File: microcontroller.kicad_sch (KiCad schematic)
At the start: 65 parts, among them IC1 MIMXRT1062DVJ6B, J3 503182-1852, J4 USB_C_pycubed, J5 JTAG_SWD_10, J6 Conn_01x06, Q6 DMG2305UX-7, SW1 KMR231NG LFS, U6 TPS54226PWPR, U7 MR25H40MDF, U8 MKL02Z32VFG4, Y1 24.0mHz, Y2 32.768kHz

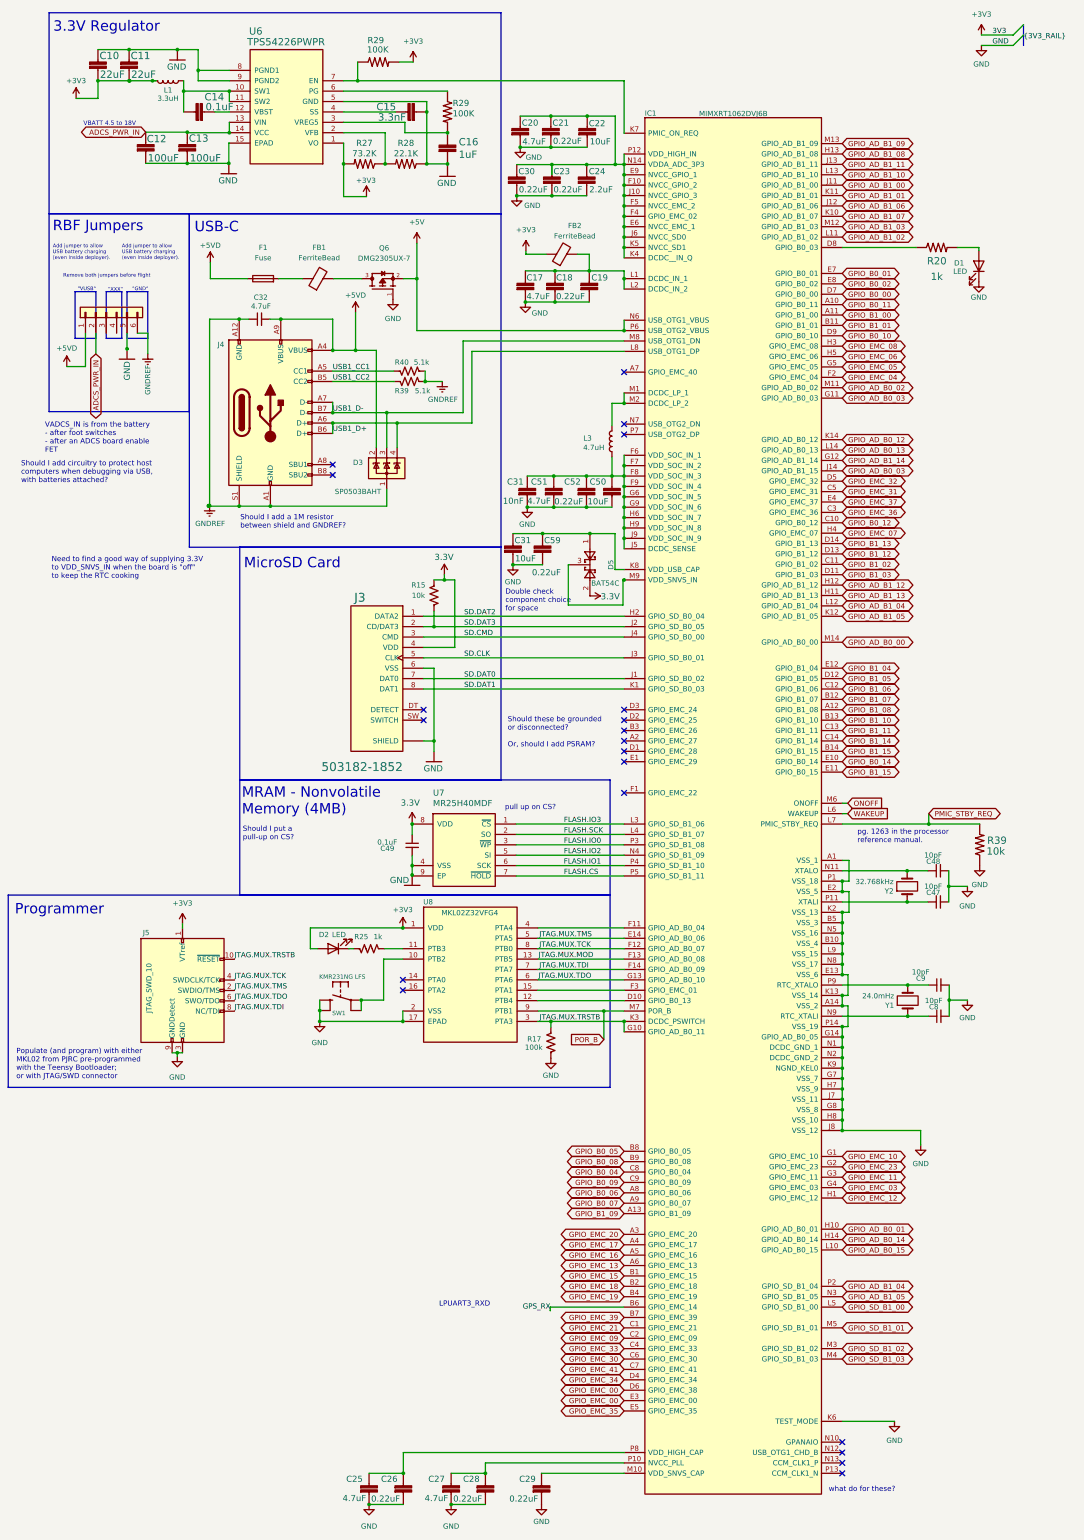
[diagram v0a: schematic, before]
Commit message: organize
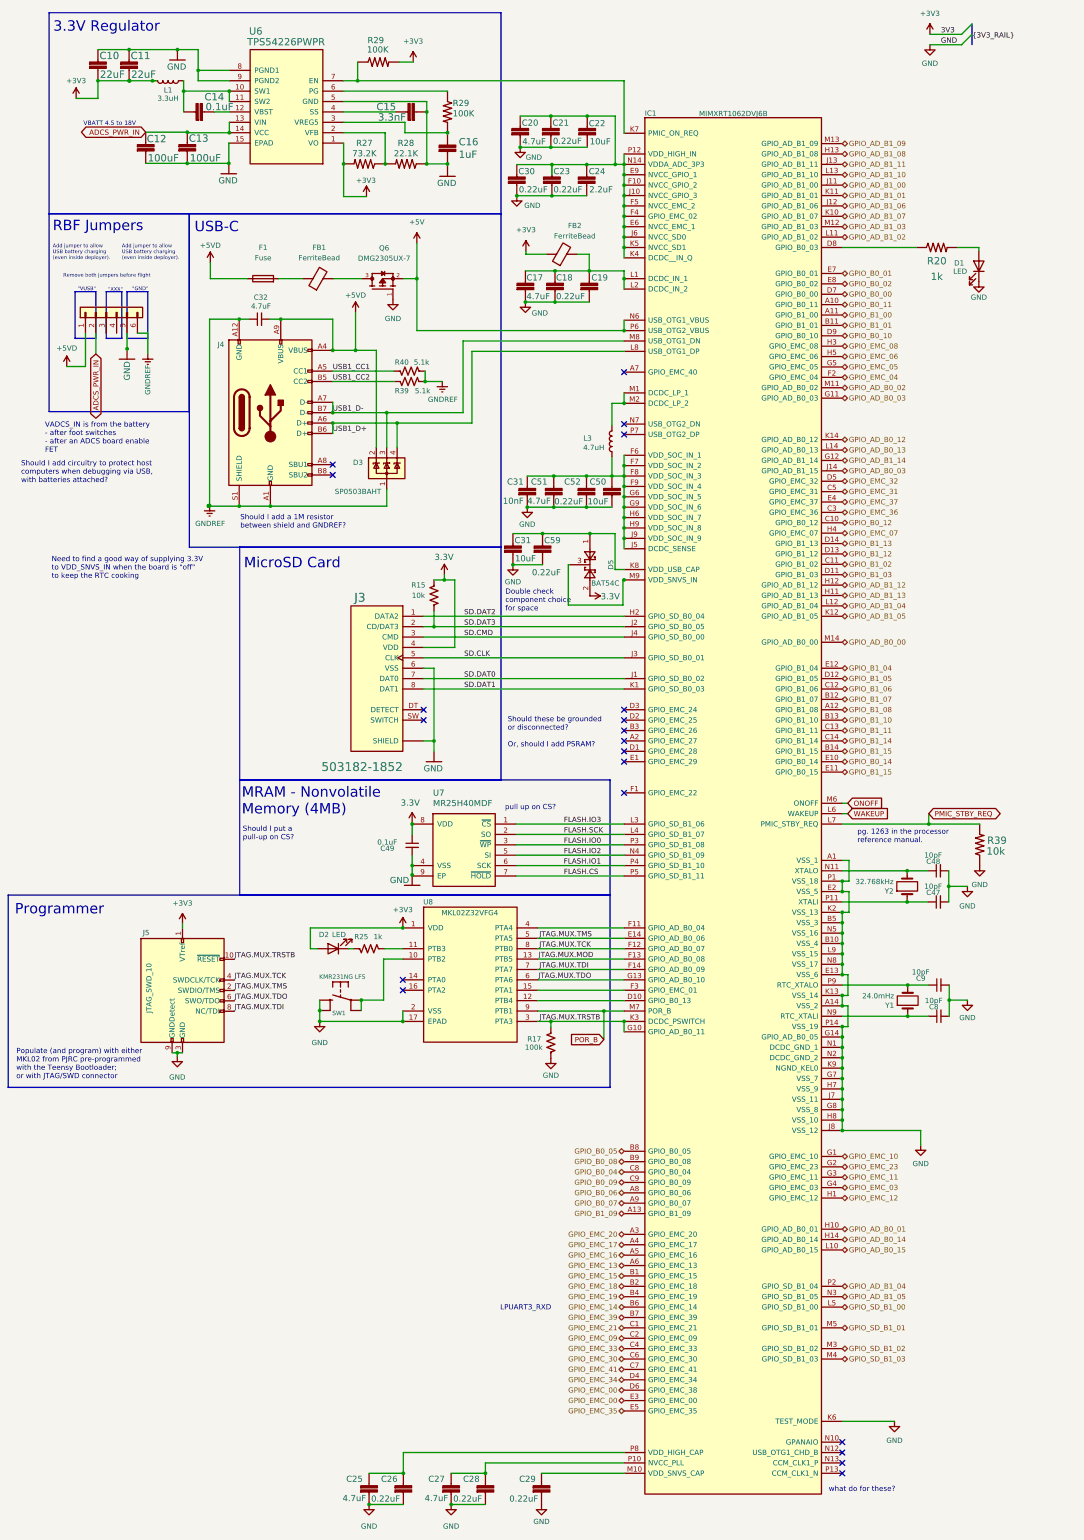
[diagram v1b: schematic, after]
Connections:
- net GPS_RX  renamed GPIO_EMC_14
